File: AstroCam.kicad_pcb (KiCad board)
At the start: 2 copper layers, 45.7 x 14 mm, 20 parts, among them P2 CONN_01X05, P3 CONN_01X10, P4 CONN_01X03, P5 CONN_01X12, P6 CONN_01X03, P7 CONN_01X03, U11 ADDI7013

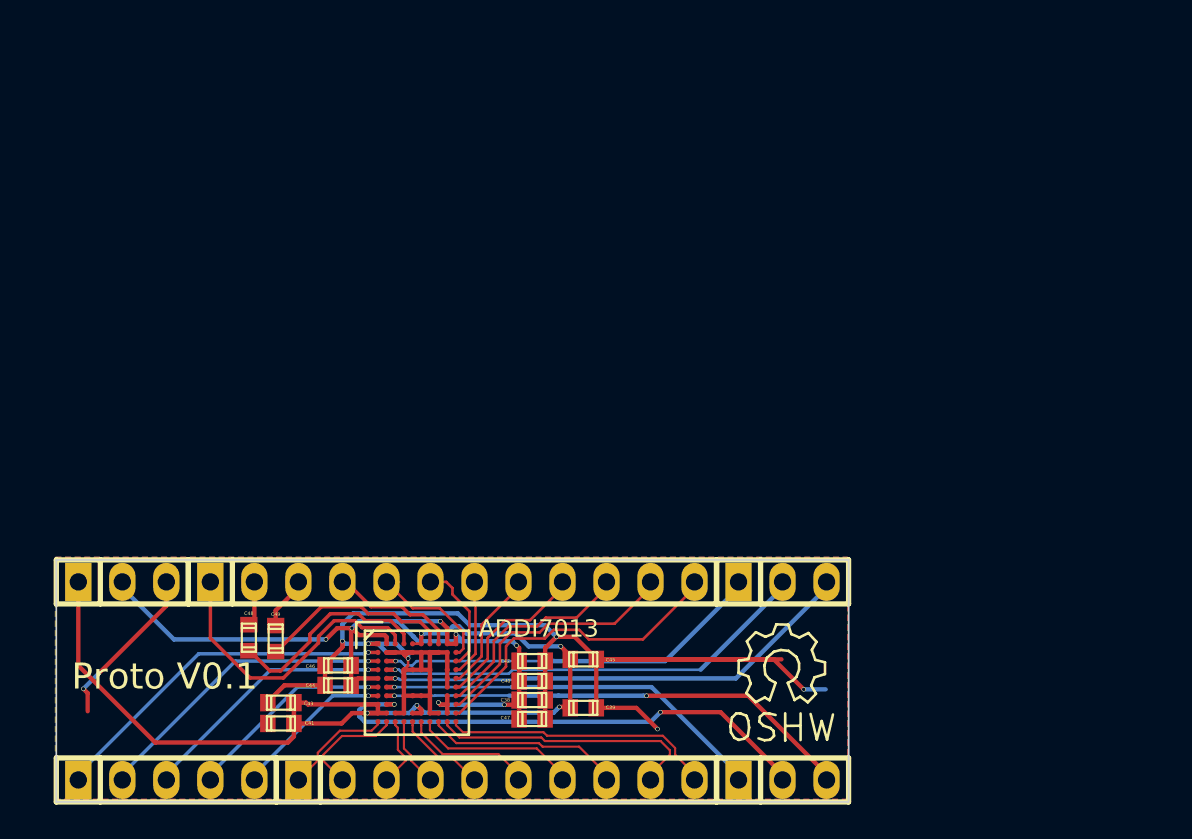
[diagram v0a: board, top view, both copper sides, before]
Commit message: Lot's of back and forward with vendor.
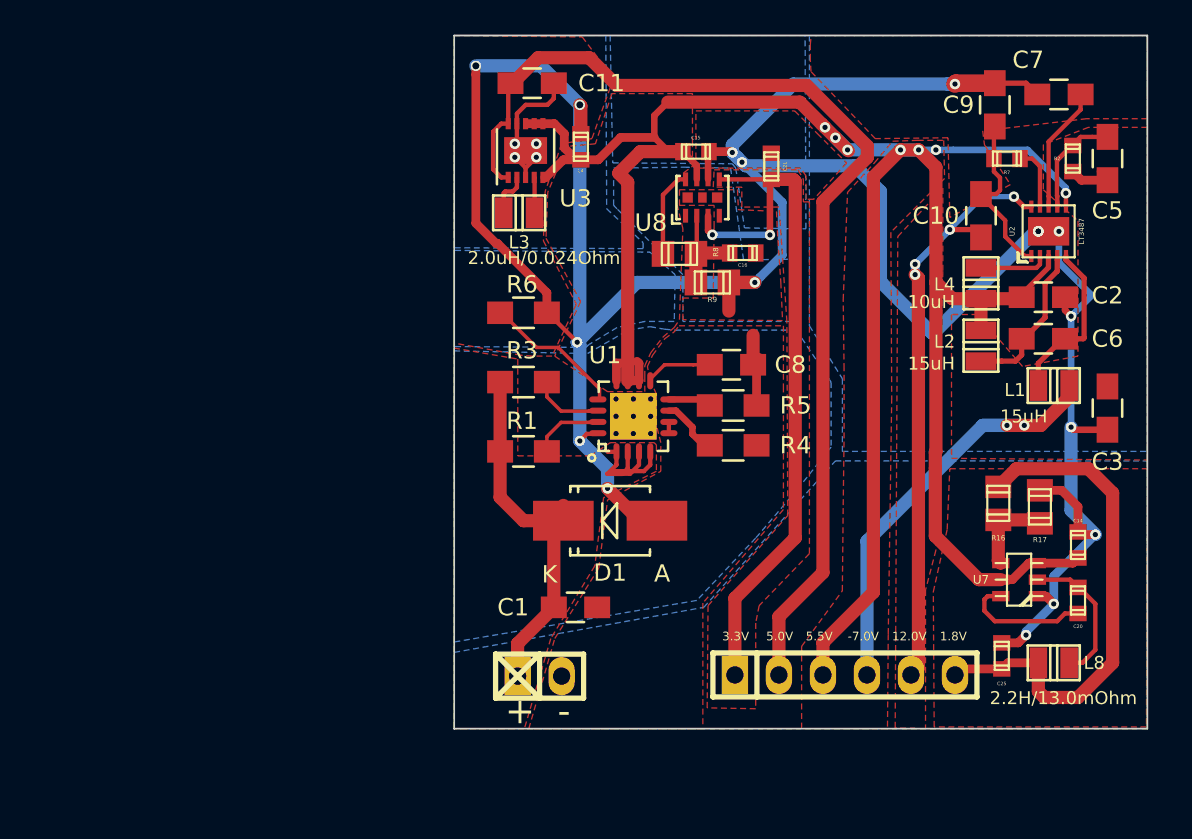
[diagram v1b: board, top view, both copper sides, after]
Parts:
- removed C38, C39, C40, C41, C42, C43, C44, C45, C46: 0.1uF, w_smd_cap:c_0603
- removed C47: 4.7uF, w_smd_cap:c_0603
- removed C48, C49: 0.1u, w_smd_cap:c_0603
- removed P2: CONN_01X05, w_pin_strip:pin_strip_5
- removed P3: CONN_01X10, w_pin_strip:pin_strip_10
- removed P4, P6, P7: CONN_01X03, w_pin_strip:pin_strip_3
- removed P5: CONN_01X12, w_pin_strip:pin_strip_12
- removed REF**: Logo, Symbols:Symbol_OSHW-Logo_SilkScreen
- removed U11: ADDI7013, camera:csp-bga-bc-76-3
- added C1: 1.0uF, Capacitors_SMD:C_0805_HandSoldering, F.Cu at (102.4, 95.6)
- added C10: 0.1uF, Capacitors_SMD:C_0805_HandSoldering, F.Cu at (125.8, 73.0)
- added C11: 10uF, Capacitors_SMD:C_0805_HandSoldering, F.Cu at (99.9, 65.3)
- added C14: 10.0F/3.0mOhm, w_smd_cap:c_0603, F.Cu at (131.4, 92.0)
- added C15: 10.0F/9Mohm, w_smd_cap:c_0603, F.Cu at (109.3, 69.3)
- added C16: 470pF, w_smd_cap:c_0603, F.Cu at (112.0, 75.2)
- added C2: 1.0uF, Capacitors_SMD:C_0805_HandSoldering, F.Cu at (129.4, 77.7)
- added C20: 100nF, w_smd_cap:c_0603, F.Cu at (131.4, 95.2)
- added C21: 10.0uF/9.0Mohm, w_smd_cap:c_0603, F.Cu at (113.7, 70.2)
- added C25: 47F/3Mohm, w_smd_cap:c_0603, F.Cu at (127.0, 98.4)
- added C3: 47pF, Capacitors_SMD:C_0805_HandSoldering, F.Cu at (133.1, 84.1)
- added C4: 2.20uF/2.80Mohm, w_smd_cap:c_0603, F.Cu at (102.7, 69.0)
- added C5: 47pF, Capacitors_SMD:C_0805_HandSoldering, F.Cu at (133.1, 69.7)
- added C6: 1.0uF, Capacitors_SMD:C_0805_HandSoldering, F.Cu at (129.4, 80.1)
- added C7: 100nF, Capacitors_SMD:C_0805_HandSoldering, F.Cu at (130.3, 66.0)
- added C8: 1.0F/11mOhm, Capacitors_SMD:C_0805_HandSoldering, F.Cu at (111.4, 81.6)
- added C9: 4.7uF, Capacitors_SMD:C_0805_HandSoldering, F.Cu at (126.6, 66.6)
- added D1: 9V/5W, Diodes_SMD:Diode-SMB_Handsoldering, F.Cu at (104.4, 90.6)
- added L1: 15uH, w_smd_inductors:inductor_smd_0805, F.Cu at (130.0, 82.8)
- added L2: 15uH, w_smd_inductors:inductor_smd_0805, F.Cu at (125.8, 80.5)
- added L3: 2.0uH/0.024Ohm, w_smd_inductors:inductor_smd_0805, F.Cu at (99.2, 72.8)
- added L4: 10uH, w_smd_inductors:inductor_smd_0805, F.Cu at (125.8, 76.9)
- added L8: 2.2H/13.0mOhm, w_smd_inductors:inductor_smd_0805, F.Cu at (130.0, 98.8)
- added P8: CONN_01X06, w_pin_strip:pin_socket_6, F.Cu at (118.0, 99.5)
- added P9: CONN_01X02, w_pin_strip:pin_socket_2, F.Cu at (100.3, 99.6)
- added R1: 10.0k, Resistors_SMD:R_0805_HandSoldering, F.Cu at (99.4, 86.6)
- added R16: 13.7k, w_smd_resistors:r_0805, F.Cu at (126.8, 89.6)
- added R17: 10.0k, w_smd_resistors:r_0805, F.Cu at (129.2, 89.8)
- added R2: 324k, w_smd_resistors:r_0603, F.Cu at (131.1, 69.7)
- added R3: 10.0k, Resistors_SMD:R_0805_HandSoldering, F.Cu at (99.4, 82.6)
- added R4: 51.1k, Resistors_SMD:R_0805_HandSoldering, F.Cu at (111.5, 86.2)
- added R5: 68.1k, Resistors_SMD:R_0805_HandSoldering, F.Cu at (111.5, 84.0)
- added R6: 53.6k, Resistors_SMD:R_0805_HandSoldering, F.Cu at (99.4, 78.6)
- added R7: 324k, w_smd_resistors:r_0603, F.Cu at (127.3, 69.7)
- added R8: 80.6k, w_smd_resistors:r_0805, F.Cu at (108.4, 75.2)
- added R9: 105k, w_smd_resistors:r_0805, F.Cu at (110.3, 76.8)
- added U1: TPS2420, camera:S-PVQFN-N16, F.Cu at (105.7, 84.6)
- added U2: LT3487, w_smd_qfn:dfn10-3x3, F.Cu at (129.7, 73.9)
- added U3: TPS63002, Housings_DFN_QFN:DFN-10-1EP_3x3mm_Pitch0.5mm, F.Cu at (99.5, 69.2)
- added U7: TPS56x200, w_smd_trans:sot23-6, F.Cu at (128.0, 94.0)
- added U8: LMZ10500, camera:llp-8, F.Cu at (109.7, 72.0)
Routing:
- net /power-supply/GND: track 0.00 -> 182.7 mm, vias 0 -> 22
- net /power-supply/5V5: track 0.00 -> 142.0 mm, vias 0 -> 7
- net /h-driver/GND: track 96.9 -> 0.00 mm, vias 8 -> 0
- net /power-supply/5V0: track 0.00 -> 63.0 mm
- net /h-driver/1V8: track 60.0 -> 0.00 mm, vias 5 -> 0
- net /h-driver/3V3: track 50.4 -> 0.00 mm, vias 7 -> 0
- net /power-supply/3V3: track 0.00 -> 42.1 mm, vias 0 -> 2
- net /power-supply/+12V: track 0.00 -> 34.5 mm, vias 0 -> 4
- net /power-supply/V_BAT: track 0.00 -> 32.1 mm
- net /h-driver/VD: track 29.6 -> 0.00 mm, vias 2 -> 0
- net /power-supply/1V8: track 0.00 -> 29.4 mm
- net /power-supply/-7V: track 0.00 -> 29.4 mm, vias 0 -> 2
- net /h-driver/SDATA: track 28.0 -> 0.00 mm, vias 1 -> 0
- net /h-driver/HD: track 27.6 -> 0.00 mm, vias 2 -> 0
- net /h-driver/SCK: track 25.3 -> 0.00 mm, vias 1 -> 0
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- added copper zone on F.Cu, net /power-supply/+12V
- added copper zone on F.Cu, net /power-supply/-7V
- added copper zone on F.Cu, net /power-supply/1V8
- added copper zone on F.Cu, net /power-supply/3V3
- added copper zone on F.Cu, net /power-supply/5V5
- added copper zone on B.Cu, net /power-supply/GND
- added copper zone on F.Cu, net /power-supply/GND
- added copper zone on B.Cu, net /power-supply/PAD
- added copper zone on F.Cu, net /power-supply/V_BAT
- removed copper zone on B.Cu, net /h-driver/GND
- removed copper zone on F.Cu, net /h-driver/GND
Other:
- board size 45.7 x 14 mm -> 40 x 40 mm
- net class Default: clearance 0.2 -> 0.1524; trace_width 0.25 -> 0.254; via_dia 0.6 -> 0.604774; via_drill 0.4 -> 0.299974
- rule trace_clearance: 0.2 -> 0.1524
- rule trace_min: 0.1 -> 0.1524
- rule via_min_drill: 0.1 -> 0.299974
- rule via_min_size: 0.1 -> 0.604774
- board text added: "+"
- board text added: "-"
- board text added: "-7.0V"
- board text added: "1.8V"
- board text added: "12.0V"
- board text added: "3.3V"
- board text added: "5.0V"
- board text added: "5.5V"
- board text removed: "Proto V0.1"
